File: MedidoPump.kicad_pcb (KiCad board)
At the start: 2 copper layers, 165.1 x 101.6 mm, 47 parts, among them J1 Flow_Fwd, J2 Flow_Rev, J3 Flow_Stop, J4 MultiplexConn, J5 OLED Disp, J6 Press_Sens, J7 MultiplexConn, J8 PwrButton, Q1 Q_NPN_EBC, SW1 SW_DPST, SW2 ~Boot, U1 BLE_FRIEND, U2 PowerButton, U3 LM7805_TO220, U4 HK3FF_RELAY, U5 ADS_1115, U6 Pololu18v17

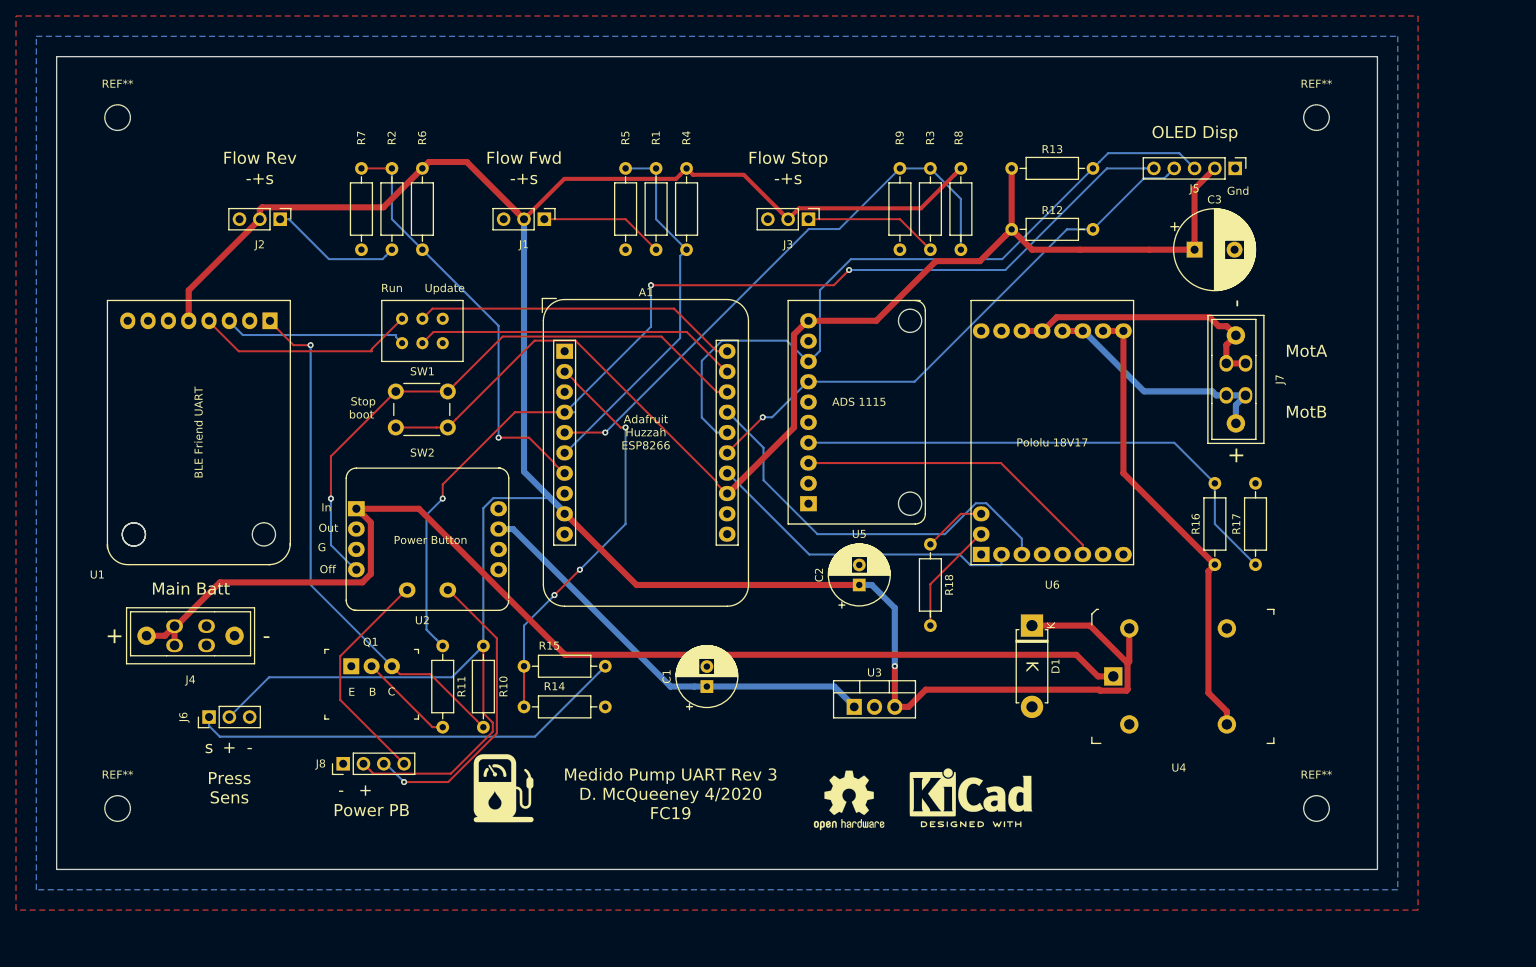
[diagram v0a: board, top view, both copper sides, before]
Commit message: misc
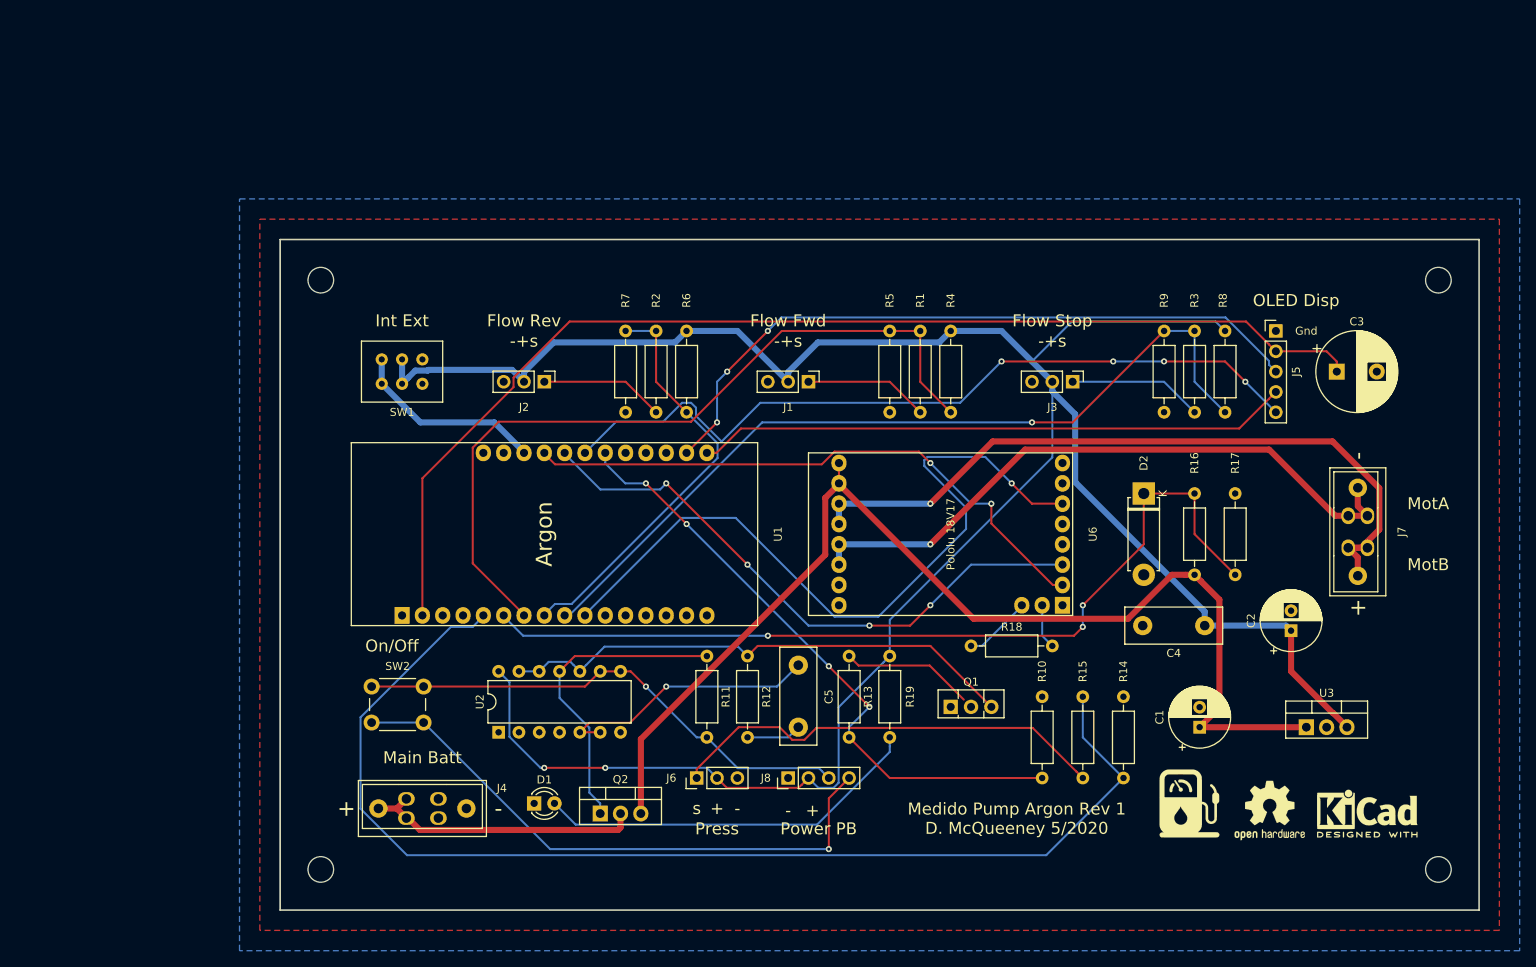
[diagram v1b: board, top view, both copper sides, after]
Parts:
- removed A1: Adafruit_HUZZAH_ESP8266_breakout, Module:Adafruit_HUZZAH_ESP8266_breakout
- removed the REF** at (134.6, 119.9)
- removed the REF** at (27.9, 35.6)
- removed the REF** at (177.8, 35.6)
- removed the REF** at (177.8, 121.9)
- removed the REF** at (27.9, 121.9)
- removed U4: HK3FF_RELAY, digikey-footprints:Relay_THT_G5LE-14
- removed U5: ADS_1115, MedidoFootprints:ADS_1115
- added ?: MountingHole_3.2mm_M3, MountingHole:MountingHole_3.2mm_M3, F.Cu at (53.3, 55.9)
- added ?: MountingHole_3.2mm_M3, MountingHole:MountingHole_3.2mm_M3, F.Cu at (193.0, 55.9)
- added ?: MountingHole_3.2mm_M3, MountingHole:MountingHole_3.2mm_M3, F.Cu at (193.0, 129.5)
- added ?: MountingHole_3.2mm_M3, MountingHole:MountingHole_3.2mm_M3, F.Cu at (53.3, 129.5)
- added C4: C, Capacitor_THT:C_Disc_D12.0mm_W4.4mm_P7.75mm, F.Cu at (163.8, 99.1)
- added C5: 0.1uF, Capacitor_THT:C_Disc_D12.0mm_W4.4mm_P7.75mm, F.Cu at (113.0, 111.8)
- added D2: 3V Zener, Diode_THT:D_5W_P10.16mm_Horizontal, F.Cu at (156.2, 82.5)
- added Q2: Q_PMOS_GDS, Package_TO_SOT_THT:TO-220-3_Vertical, F.Cu at (88.3, 122.6)
- added R19: 330R, Resistor_THT:R_Axial_DIN0207_L6.3mm_D2.5mm_P10.16mm_Horizontal, F.Cu at (124.5, 113.0)
- added REF**: KiCad-Logo2_5mm_SilkScreen, Symbol:KiCad-Logo2_5mm_SilkScreen, F.Cu at (184.2, 122.6)
- D1: value D -> Power; footprint Diode_THT:D_5W_P10.16mm_Horizontal -> LED_THT:LED_D3.0mm
- Q1: value Q_NPN_EBC -> 2N3904; footprint digikey-footprints:SIP-3_P2.54mm -> Package_TO_SOT_THT:TO-126-3_Vertical
- R11: value 47K -> 100K
- R12: value 4K7 -> 100K
- R13: value 4K7 -> 1K
- R14: value 4K7 -> 33K
- R17: value 3K3 -> 6K8
- SW2: value ~Boot -> On/Off
- U1: value BLE_FRIEND -> Particle_Argon; footprint MedidoFootprints:BLE_FRIEND -> MedidoFootprints:Particle_Argon
- U2: value PowerButton -> HEF4093B; footprint MedidoFootprints:PowerButton -> Package_DIP:DIP-14_W7.62mm
- moved G*** 85.7 mm to (161.9, 121.3)
- moved R14 75.5 mm to (153.7, 118.1), turned to 90 degrees
- moved Q1 75.1 mm to (132.1, 109.2)
- moved R10 71.8 mm to (143.5, 118.1), turned to 90 degrees
- moved D1 66.1 mm to (80.0, 121.3), turned to 0 degrees
- moved R13 64.3 mm to (119.4, 102.9), turned to 270 degrees
- moved R12 62.7 mm to (106.7, 102.9), turned to 270 degrees
- moved C1 61.8 mm to (163.2, 111.8)
- moved J6 61.4 mm to (100.3, 118.1)
- moved R15 61.3 mm to (148.6, 118.1), turned to 90 degrees
- moved U3 56.6 mm to (176.5, 111.8)
- moved J8 55.7 mm to (111.8, 118.1)
- moved C2 54.3 mm to (174.6, 99.7)
- moved U1 52.9 mm to (83.8, 87.6), turned to 90 degrees
- moved REF** 52.6 mm to (172.0, 122.2)
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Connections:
- D1 pad 1: +5V -> GND
- D1 pad 2: GND -> Net-(D1-Pad2)
- J5 pad 3: Net-(A1-Pad16) -> Net-(J5-Pad3)
- J5 pad 4: Net-(A1-Pad15) -> Net-(J5-Pad4)
- J5 pad 5: /OLED_RST -> Net-(J5-Pad5)
- R1 pad 1: Net-(A1-Pad6) -> Net-(R1-Pad1)
- R10 pad 1: +5V -> Net-(R10-Pad1)
- R10 pad 2: Net-(Q1-Pad3) -> GND
- R11 pad 1: /OLED_RST -> Net-(Q2-Pad1)
- R11 pad 2: Net-(Q1-Pad2) -> Net-(J8-Pad3)
- R12 pad 1: +3V3 -> Net-(Q1-Pad3)
- R12 pad 2: Net-(A1-Pad15) -> Net-(C5-Pad1)
- R13 pad 1: +3V3 -> Net-(Q1-Pad2)
- R13 pad 2: Net-(A1-Pad16) -> Net-(R10-Pad1)
- R14 pad 1: Net-(A1-Pad2) -> Net-(R14-Pad1)
- R15 pad 2: Net-(A1-Pad2) -> Net-(R14-Pad1)
- R16 pad 1: Net-(R16-Pad1) -> Net-(C1-Pad1)
- R16 pad 2: Net-(R16-Pad2) -> Net-(D2-Pad1)
- R17 pad 1: Net-(R16-Pad2) -> Net-(D2-Pad1)
- R2 pad 1: Net-(A1-Pad7) -> Net-(R2-Pad1)
- R3 pad 1: Net-(A1-Pad5) -> Net-(R3-Pad1)
- R4 pad 2: Net-(A1-Pad6) -> Net-(R1-Pad1)
- R5 pad 1: Net-(A1-Pad6) -> Net-(R1-Pad1)
- R6 pad 2: Net-(A1-Pad7) -> Net-(R2-Pad1)
- R7 pad 1: Net-(A1-Pad7) -> Net-(R2-Pad1)
- R8 pad 2: Net-(A1-Pad5) -> Net-(R3-Pad1)
- R9 pad 1: Net-(A1-Pad5) -> Net-(R3-Pad1)
- SW1 pad 2: Net-(A1-Pad19) -> +5V
- SW1 pad 3: Net-(SW1-Pad3) -> Net-(SW1-Pad1)
- SW1 pad 4: Net-(A1-Pad20) -> +5V
- SW2 pad 1: +3V3 -> Net-(J8-Pad3)
- SW2 pad 2: Net-(A1-Pad18) -> Net-(J8-Pad4)
- U1 pad 1: Net-(Q1-Pad3) -> Net-(U1-Pad1)
- U1 pad 2: GND -> +3V3
- U1 pad 3: Net-(SW1-Pad1) -> Net-(U1-Pad3)
- U1 pad 4: Net-(SW1-Pad3) -> GND
- U1 pad 5: +5V -> Net-(R14-Pad1)
- U1 pad 6: Net-(U1-Pad6) -> Net-(D2-Pad1)
- U1 pad 7: GND -> Net-(R1-Pad1)
- U1 pad 8: Net-(U1-Pad8) -> Net-(R2-Pad1)
- U2 pad 1: Net-(J4-Pad4) -> GND
- U2 pad 10: Net-(J8-Pad4) -> Net-(Q1-Pad3)
- U2 pad 2: Net-(U2-Pad2) -> GND
- U2 pad 3: GND -> Net-(U2-Pad3)
- U2 pad 4: Net-(A1-Pad18) -> Net-(U2-Pad4)
- U2 pad 5: Net-(U2-Pad5) -> GND
- U2 pad 6: Net-(U2-Pad6) -> GND
- U2 pad 7: Net-(C1-Pad1) -> Net-(U2-Pad7)
- U2 pad 8: Net-(U2-Pad8) -> Net-(J8-Pad3)
- U6 pad 10: Net-(R16-Pad1) -> Net-(C1-Pad1)
- U6 pad 2: Net-(A1-Pad14) -> Net-(U1-Pad25)
- U6 pad 3: Net-(A1-Pad17) -> Net-(U1-Pad24)
- U6 pad 6: Net-(U5-Pad3) -> Net-(U1-Pad10)
- U6 pad 9: Net-(R16-Pad1) -> Net-(C1-Pad1)
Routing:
- net Net-(R14-Pad1): track 0.00 -> 146.1 mm
- net /OLED_RST: track 131.5 -> 0.00 mm, vias 3 -> 0
- net Net-(D2-Pad1): track 0.00 -> 112.4 mm, vias 0 -> 3
- net Net-(J4-Pad4): track 146.1 -> 35.0 mm
- net Net-(R3-Pad1): track 0.00 -> 105.2 mm, vias 0 -> 1
- net Net-(J5-Pad5): track 0.00 -> 98.3 mm, vias 0 -> 4
- net Net-(R1-Pad1): track 0.00 -> 97.3 mm
- net Net-(U1-Pad10): track 0.00 -> 93.0 mm, vias 0 -> 1
- net Net-(A1-Pad16): track 90.8 -> 0.00 mm
- net Net-(C1-Pad1): track 53.7 -> 142.5 mm
- net Net-(J5-Pad3): track 0.00 -> 86.7 mm, vias 0 -> 3
- net Net-(R10-Pad1): track 0.00 -> 78.0 mm, vias 0 -> 4
- net Net-(U1-Pad24): track 0.00 -> 75.0 mm, vias 0 -> 4
- net Net-(U1-Pad25): track 0.00 -> 74.4 mm, vias 0 -> 2
- net Net-(J5-Pad4): track 0.00 -> 74.3 mm
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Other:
- board size 165.1 x 101.6 mm -> 149.9 x 83.8 mm
- board text added: "Int Ext"
- board text added: "Medido Pump Argon Rev 1 D. McQueeney 5/2020"
- board text added: "On/Off"
- board text added: "Press"
- board text removed: "Adafruit Huzzah ESP8266"
- board text removed: "B"
- board text removed: "C"
- board text removed: "E"
- board text removed: "G"
- board text removed: "In"
- board text removed: "K"
- board text removed: "Medido Pump UART Rev 3 D. McQueeney 4/2020 FC19"
- board text removed: "Off"
- board text removed: "Out"
- board text removed: "Press Sens"
- board text removed: "Run"
- board text removed: "Stop boot"
- board text removed: "Update"
